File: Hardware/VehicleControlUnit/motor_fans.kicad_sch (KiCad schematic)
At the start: 12 parts

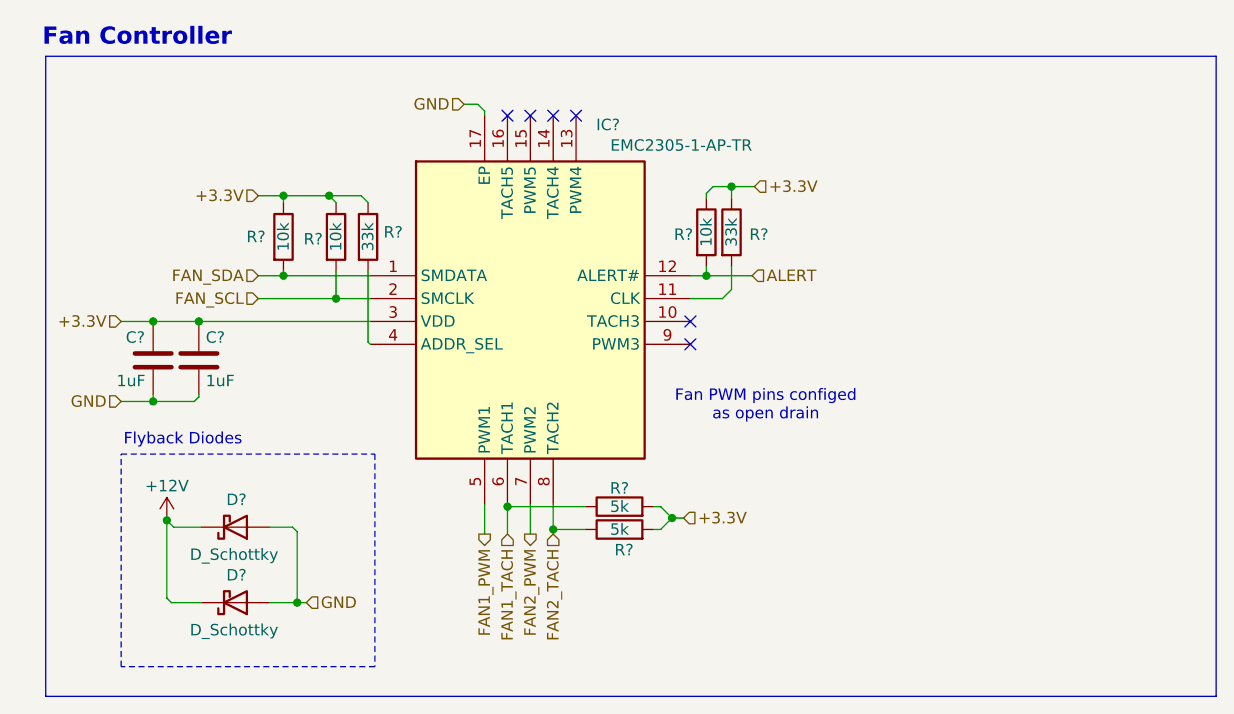
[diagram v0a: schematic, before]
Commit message: VCU more like diddle-u, mika time
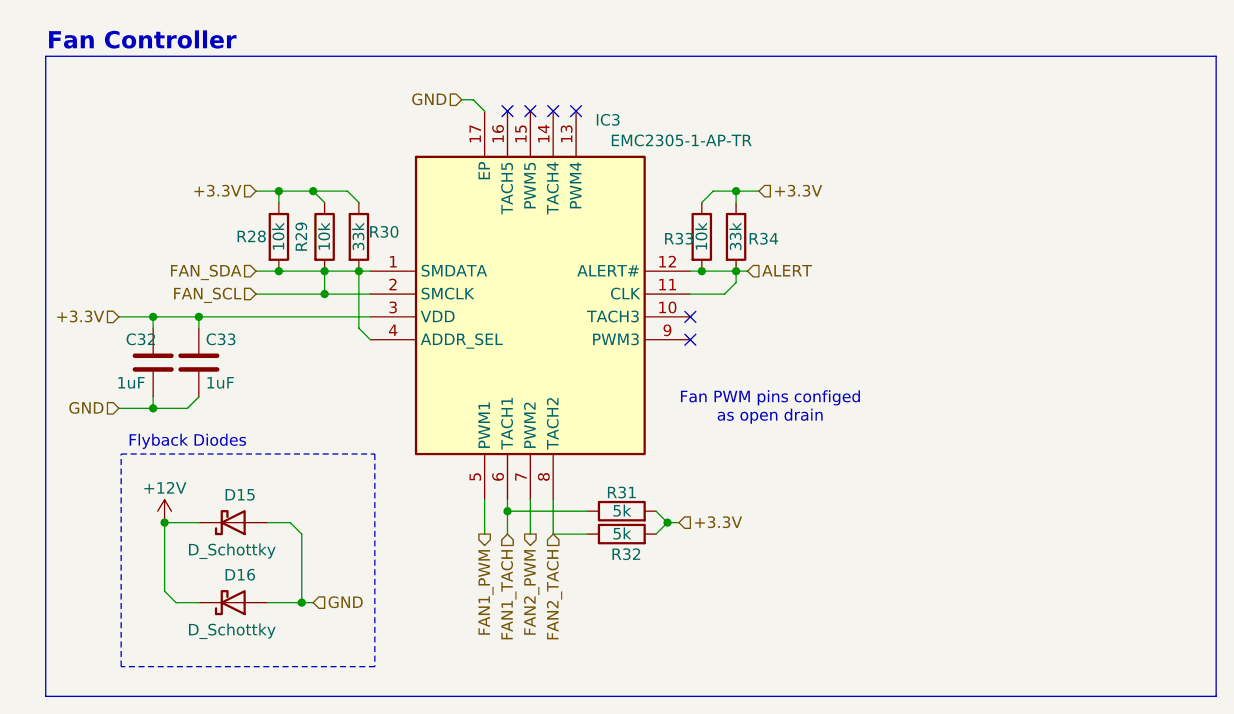
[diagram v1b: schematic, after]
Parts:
- gave numbers to parts that had none: 12
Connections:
- net FAN_SDA is gone; now on net FAN_SCL: IC3.1 (SMDATA), R28.2
- net ALERT: now also IC3.11 (CLK), R34.2
- net FAN_SCL: now also IC3.4 (ADDR_SEL), R30.2
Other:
- moved on the sheet: D15, IC3, R28, R29, R30, R31, R32, R33, R34

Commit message: mika changes
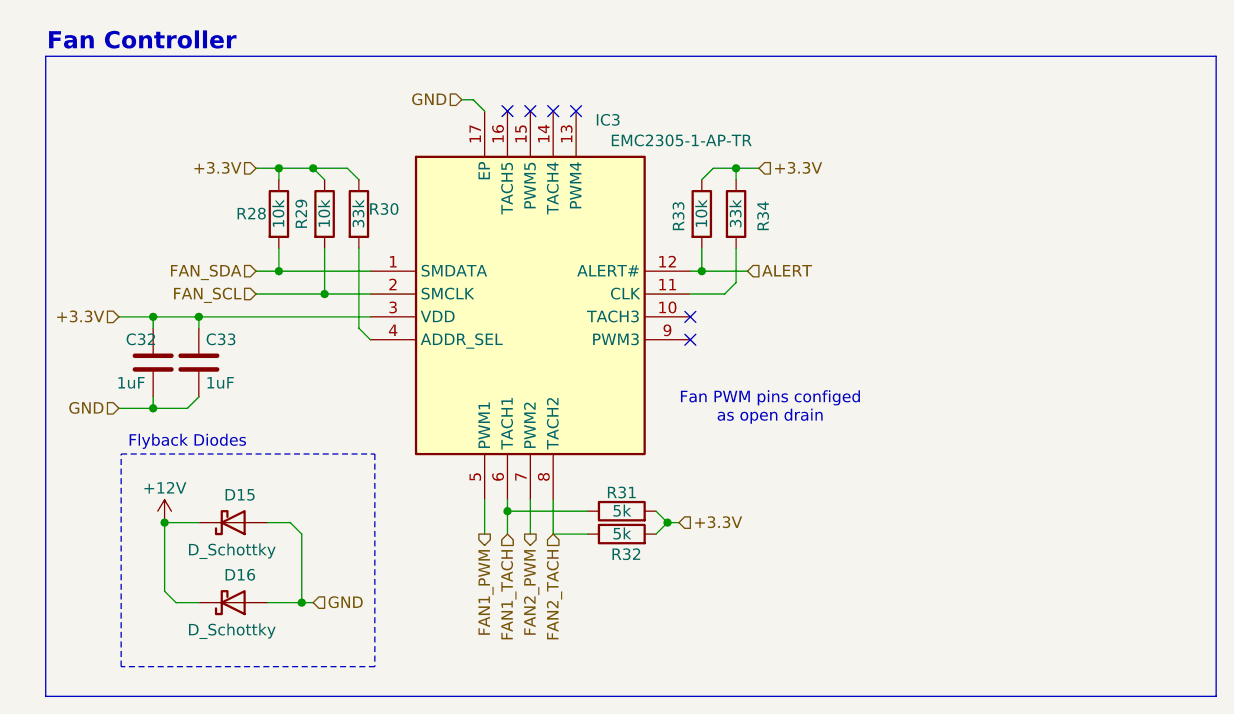
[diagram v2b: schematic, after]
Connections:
- net ALERT: no longer IC3.11 (CLK), R34.2
- net FAN_SCL: no longer IC3.1 (SMDATA), IC3.4 (ADDR_SEL), R28.2, R30.2
- new net: IC3.11 (CLK), R34.2
- new net: IC3.4 (ADDR_SEL), R30.2
- new net FAN_SDA: IC3.1 (SMDATA), R28.2
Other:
- moved on the sheet: R28, R29, R30, R33, R34
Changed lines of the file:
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@@
 	)
 	(junction
-		(at 66.04 40.64)
+		(at 66.04 38.1)
 		(diameter 0)
 		(color 0 0 0 0)
 	)
 	(junction
-		(at 71.12 49.53)
+		(at 66.04 49.53)
 		(diameter 0)
 		(color 0 0 0 0)
@@
 	)
 	(junction
-		(at 113.03 49.53)
-		(diameter 0)
-		(color 0 0 0 0)
-	)
-	(junction
 		(at 109.22 77.47)
 		(diameter 0)
@@
 	)
 	(junction
-		(at 69.85 40.64)
-		(diameter 0)
-		(color 0 0 0 0)
-	)
-	(junction
-		(at 71.12 52.07)
+		(at 113.03 49.53)
 		(diameter 0)
 		(color 0 0 0 0)
 	)
 	(junction
-		(at 66.04 49.53)
+		(at 69.85 38.1)
 		(diameter 0)
 		(color 0 0 0 0)
 	)
 	(junction
-		(at 91.44 76.2)
+		(at 71.12 52.07)
 		(diameter 0)
 		(color 0 0 0 0)
@@
 	)
 	(junction
-		(at 74.93 49.53)
-		(diameter 0)
-		(color 0 0 0 0)
-	)
-	(junction
-		(at 116.84 49.53)
+		(at 91.44 76.2)
 		(diameter 0)
 		(color 0 0 0 0)
 	)
 	(junction
-		(at 116.84 40.64)
+		(at 116.84 38.1)
 		(diameter 0)
 		(color 0 0 0 0)
@@
 	(wire
 		(pts
-			(xy 71.12 41.91) (xy 69.85 40.64)
+			(xy 71.12 39.37) (xy 69.85 38.1)
 		)
 		(stroke
@@
 	(wire
 		(pts
-			(xy 71.12 49.53) (xy 74.93 49.53)
+			(xy 66.04 49.53) (xy 76.2 49.53)
 		)
 		(stroke
@@
 	(wire
 		(pts
-			(xy 63.5 40.64) (xy 66.04 40.64)
+			(xy 66.04 46.99) (xy 66.04 49.53)
+		)
+		(stroke
+			(width 0)
+			(type default)
+		)
+	)
+	(wire
+		(pts
+			(xy 63.5 38.1) (xy 66.04 38.1)
 		)
 		(stroke
@@
 	(wire
 		(pts
-			(xy 116.84 49.53) (xy 118.11 49.53)
+			(xy 113.03 49.53) (xy 118.11 49.53)
 		)
 		(stroke
@@
 	(wire
 		(pts
-			(xy 74.93 49.53) (xy 76.2 49.53)
-		)
-		(stroke
-			(width 0)
-			(type default)
-		)
-	)
-	(wire
-		(pts
 			(xy 64.77 77.47) (xy 67.31 77.47)
 		)
@@
 	(wire
 		(pts
-			(xy 69.85 40.64) (xy 73.66 40.64)
+			(xy 69.85 38.1) (xy 73.66 38.1)
 		)
 		(stroke
@@
 	(wire
 		(pts
-			(xy 114.3 40.64) (xy 116.84 40.64)
+			(xy 114.3 38.1) (xy 116.84 38.1)
 		)
 		(stroke
@@
 	(wire
 		(pts
-			(xy 113.03 49.53) (xy 116.84 49.53)
-		)
-		(stroke
-			(width 0)
-			(type default)
-		)
-	)
-	(wire
-		(pts
 			(xy 93.98 78.74) (xy 93.98 74.93)
 		)
@@
 	(wire
 		(pts
-			(xy 113.03 41.91) (xy 114.3 40.64)
+			(xy 113.03 39.37) (xy 114.3 38.1)
 		)
 		(stroke
@@
 	(wire
 		(pts
-			(xy 74.93 49.53) (xy 74.93 55.88)
-		)
-		(stroke
-			(width 0)
-			(type default)
-		)
-	)
-	(wire
-		(pts
-			(xy 66.04 40.64) (xy 69.85 40.64)
+			(xy 74.93 46.99) (xy 74.93 55.88)
 		)
 		(stroke
@@
 	(wire
 		(pts
-			(xy 66.04 49.53) (xy 71.12 49.53)
+			(xy 66.04 38.1) (xy 69.85 38.1)
 		)
 		(stroke
@@
 	(wire
 		(pts
-			(xy 116.84 40.64) (xy 119.38 40.64)
+			(xy 116.84 38.1) (xy 119.38 38.1)
 		)
 		(stroke
@@
 	(wire
 		(pts
-			(xy 66.04 40.64) (xy 66.04 41.91)
+			(xy 66.04 38.1) (xy 66.04 39.37)
 		)
 		(stroke
@@
 	(wire
 		(pts
-			(xy 116.84 49.53) (xy 116.84 50.8)
+			(xy 116.84 46.99) (xy 116.84 50.8)
 		)
 		(stroke
@@
 	(wire
 		(pts
-			(xy 71.12 49.53) (xy 71.12 52.07)
+			(xy 71.12 46.99) (xy 71.12 52.07)
 		)
 		(stroke
@@
 	(wire
 		(pts
-			(xy 74.93 41.91) (xy 73.66 40.64)
+			(xy 74.93 39.37) (xy 73.66 38.1)
 		)
 		(stroke
@@
 	(wire
 		(pts
-			(xy 116.84 40.64) (xy 116.84 41.91)
+			(xy 116.84 38.1) (xy 116.84 39.37)
 		)
 		(stroke
@@
 	(wire
 		(pts
+			(xy 113.03 46.99) (xy 113.03 49.53)
+		)
+		(stroke
+			(width 0)
+			(type default)
+		)
+	)
+	(wire
+		(pts
 			(xy 111.76 49.53) (xy 113.03 49.53)
 		)
@@
 	(hierarchical_label "+3.3V"
 		(shape input)
-		(at 63.5 40.64 180)
+		(at 63.5 38.1 180)
 		(effects
 			(font
@@
 	(hierarchical_label "+3.3V"
 		(shape input)
-		(at 119.38 40.64 0)
+		(at 119.38 38.1 0)
 		(effects
 			(font
@@
 	(symbol
 		(lib_id "Device:R")
-		(at 66.04 45.72 0)
+		(at 66.04 43.18 0)
 		(unit 1)
 		(body_style 1)
@@
 		(dnp no)
 		(property "Reference" "R28"
-			(at 62.992 45.72 0)
+			(at 62.992 43.18 0)
 			(show_name no)
 			(do_not_autoplace no)
@@
 		)
 		(property "Value" "10k"
-			(at 66.04 45.72 90)
+			(at 66.04 43.18 90)
 			(show_name no)
 			(do_not_autoplace no)
@@
 		)
 		(property "Footprint" ""
-			(at 64.262 45.72 90)
+			(at 64.262 43.18 90)
 			(hide yes)
 			(show_name no)
@@
 		)
 		(property "Datasheet" ""
-			(at 66.04 45.72 0)
+			(at 66.04 43.18 0)
 			(hide yes)
 			(show_name no)
@@
 		)
 		(property "Description" "Resistor"
-			(at 66.04 45.72 0)
+			(at 66.04 43.18 0)
 			(hide yes)
 			(show_name no)
@@
 	(symbol
 		(lib_id "Device:R")
-		(at 113.03 45.72 0)
+		(at 113.03 43.18 0)
 		(unit 1)
 		(body_style 1)
@@
 		(dnp no)
 		(property "Reference" "R33"
-			(at 110.49 45.974 0)
+			(at 110.49 43.434 90)
 			(show_name no)
 			(do_not_autoplace no)
@@
 		)
 		(property "Value" "10k"
-			(at 113.03 45.72 90)
+			(at 113.03 43.18 90)
 			(show_name no)
 			(do_not_autoplace no)
@@
 		)
 		(property "Footprint" ""
-			(at 111.252 45.72 90)
+			(at 111.252 43.18 90)
 			(hide yes)
 			(show_name no)
@@
 		)
 		(property "Datasheet" ""
-			(at 113.03 45.72 0)
+			(at 113.03 43.18 0)
 			(hide yes)
 			(show_name no)
@@
 		)
 		(property "Description" "Resistor"
-			(at 113.03 45.72 0)
+			(at 113.03 43.18 0)
 			(hide yes)
 			(show_name no)
@@
 	(symbol
 		(lib_id "Device:R")
-		(at 116.84 45.72 0)
+		(at 116.84 43.18 0)
 		(unit 1)
 		(body_style 1)
@@
 		(dnp no)
 		(property "Reference" "R34"
-			(at 119.888 45.974 0)
+			(at 119.888 43.434 90)
 			(show_name no)
 			(do_not_autoplace no)
@@
 		)
 		(property "Value" "33k"
-			(at 116.84 45.72 90)
+			(at 116.84 43.18 90)
 			(show_name no)
 			(do_not_autoplace no)
@@
 		)
 		(property "Footprint" ""
-			(at 115.062 45.72 90)
+			(at 115.062 43.18 90)
 			(hide yes)
 			(show_name no)
@@
 		)
 		(property "Datasheet" ""
-			(at 116.84 45.72 0)
+			(at 116.84 43.18 0)
 			(hide yes)
 			(show_name no)
@@
 		)
 		(property "Description" "Resistor"
-			(at 116.84 45.72 0)
+			(at 116.84 43.18 0)
 			(hide yes)
 			(show_name no)
@@
 	(symbol
 		(lib_id "Device:R")
-		(at 71.12 45.72 0)
+		(at 71.12 43.18 0)
 		(unit 1)
 		(body_style 1)
@@
 		(dnp no)
 		(property "Reference" "R29"
-			(at 68.58 45.72 90)
+			(at 68.58 43.18 90)
 			(show_name no)
 			(do_not_autoplace no)
@@
 		)
 		(property "Value" "10k"
-			(at 71.12 45.72 90)
+			(at 71.12 43.18 90)
 			(show_name no)
 			(do_not_autoplace no)
@@
 		)
 		(property "Footprint" ""
-			(at 69.342 45.72 90)
+			(at 69.342 43.18 90)
 			(hide yes)
 			(show_name no)
@@
 		)
 		(property "Datasheet" ""
-			(at 71.12 45.72 0)
+			(at 71.12 43.18 0)
 			(hide yes)
 			(show_name no)
@@
 		)
 		(property "Description" "Resistor"
-			(at 71.12 45.72 0)
+			(at 71.12 43.18 0)
 			(hide yes)
 			(show_name no)
@@
 	(symbol
 		(lib_id "Device:R")
-		(at 74.93 45.72 0)
+		(at 74.93 43.18 0)
 		(unit 1)
 		(body_style 1)
@@
 		(dnp no)
 		(property "Reference" "R30"
-			(at 77.724 45.212 0)
+			(at 77.724 42.672 0)
 			(show_name no)
 			(do_not_autoplace no)
@@
 		)
 		(property "Value" "33k"
-			(at 74.93 45.72 90)
+			(at 74.93 43.18 90)
 			(show_name no)
 			(do_not_autoplace no)
@@
 		)
 		(property "Footprint" ""
-			(at 73.152 45.72 90)
+			(at 73.152 43.18 90)
 			(hide yes)
 			(show_name no)
@@
 		)
 		(property "Datasheet" ""
-			(at 74.93 45.72 0)
+			(at 74.93 43.18 0)
 			(hide yes)
 			(show_name no)
@@
 		)
 		(property "Description" "Resistor"
-			(at 74.93 45.72 0)
+			(at 74.93 43.18 0)
 			(hide yes)
 			(show_name no)
